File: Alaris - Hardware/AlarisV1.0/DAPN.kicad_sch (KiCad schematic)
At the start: 35 parts, among them J1 MSD-1-A, J4 Header 4x2, J5 MSD-1-A, SW3 SW_MEC_5G, SW4 SW_MEC_5G, U13 STM32H723VGTx, Y6 32k768, Y7 25MHz

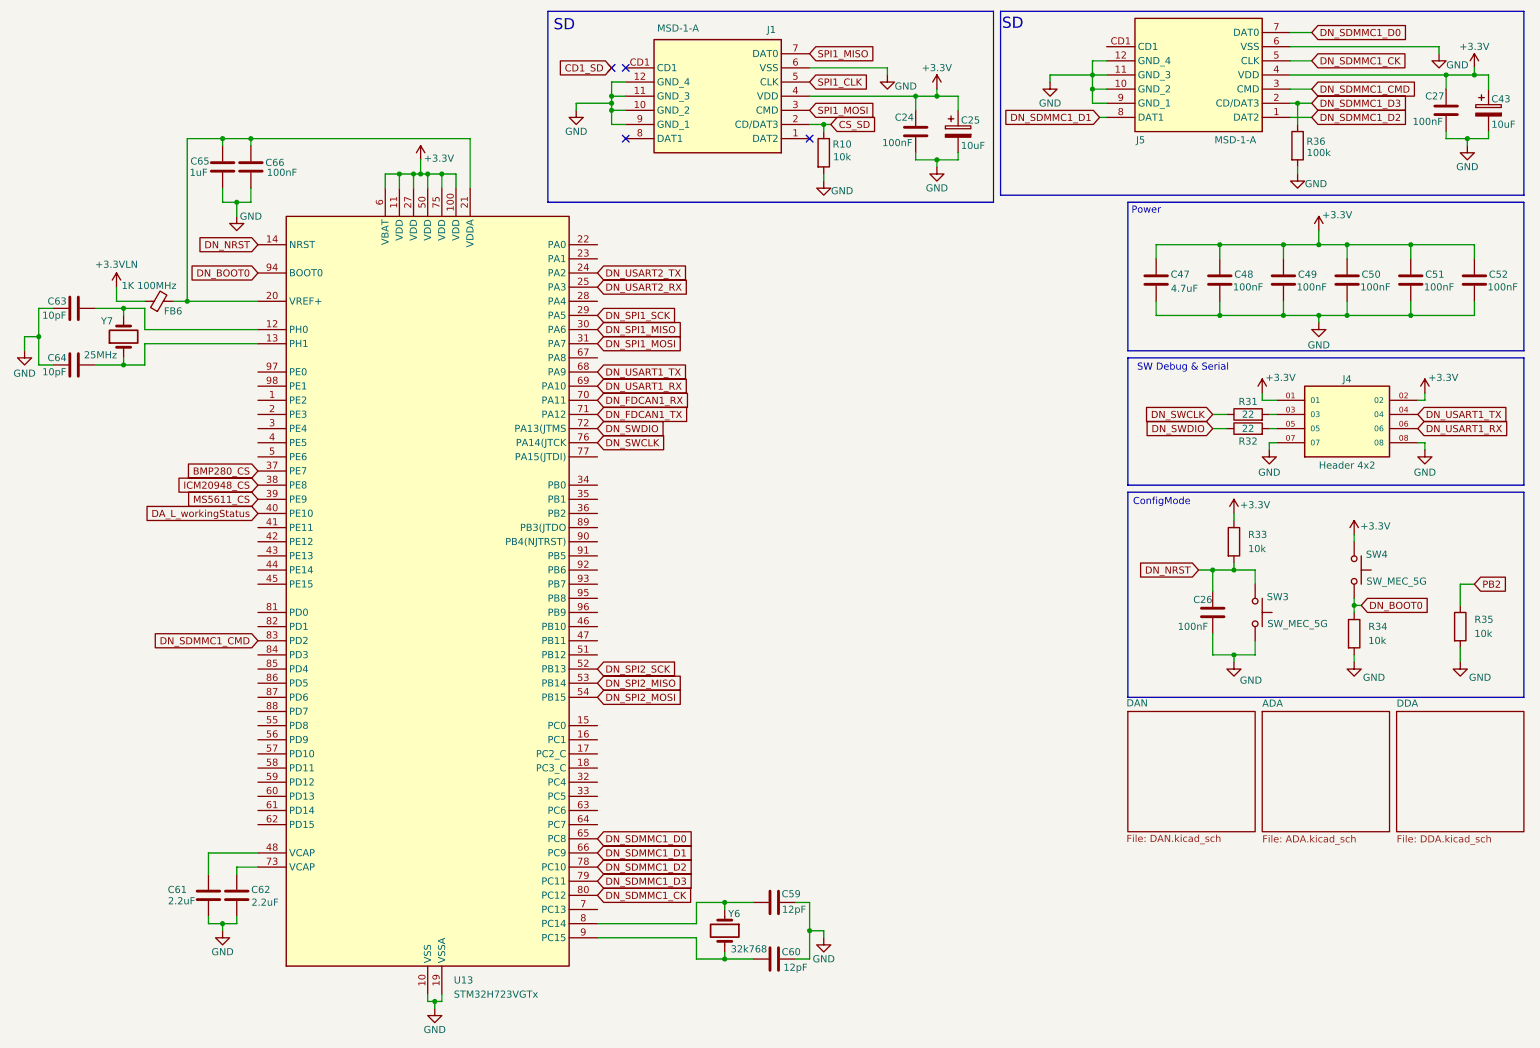
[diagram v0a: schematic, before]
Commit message: Desenvolvimento da PCB
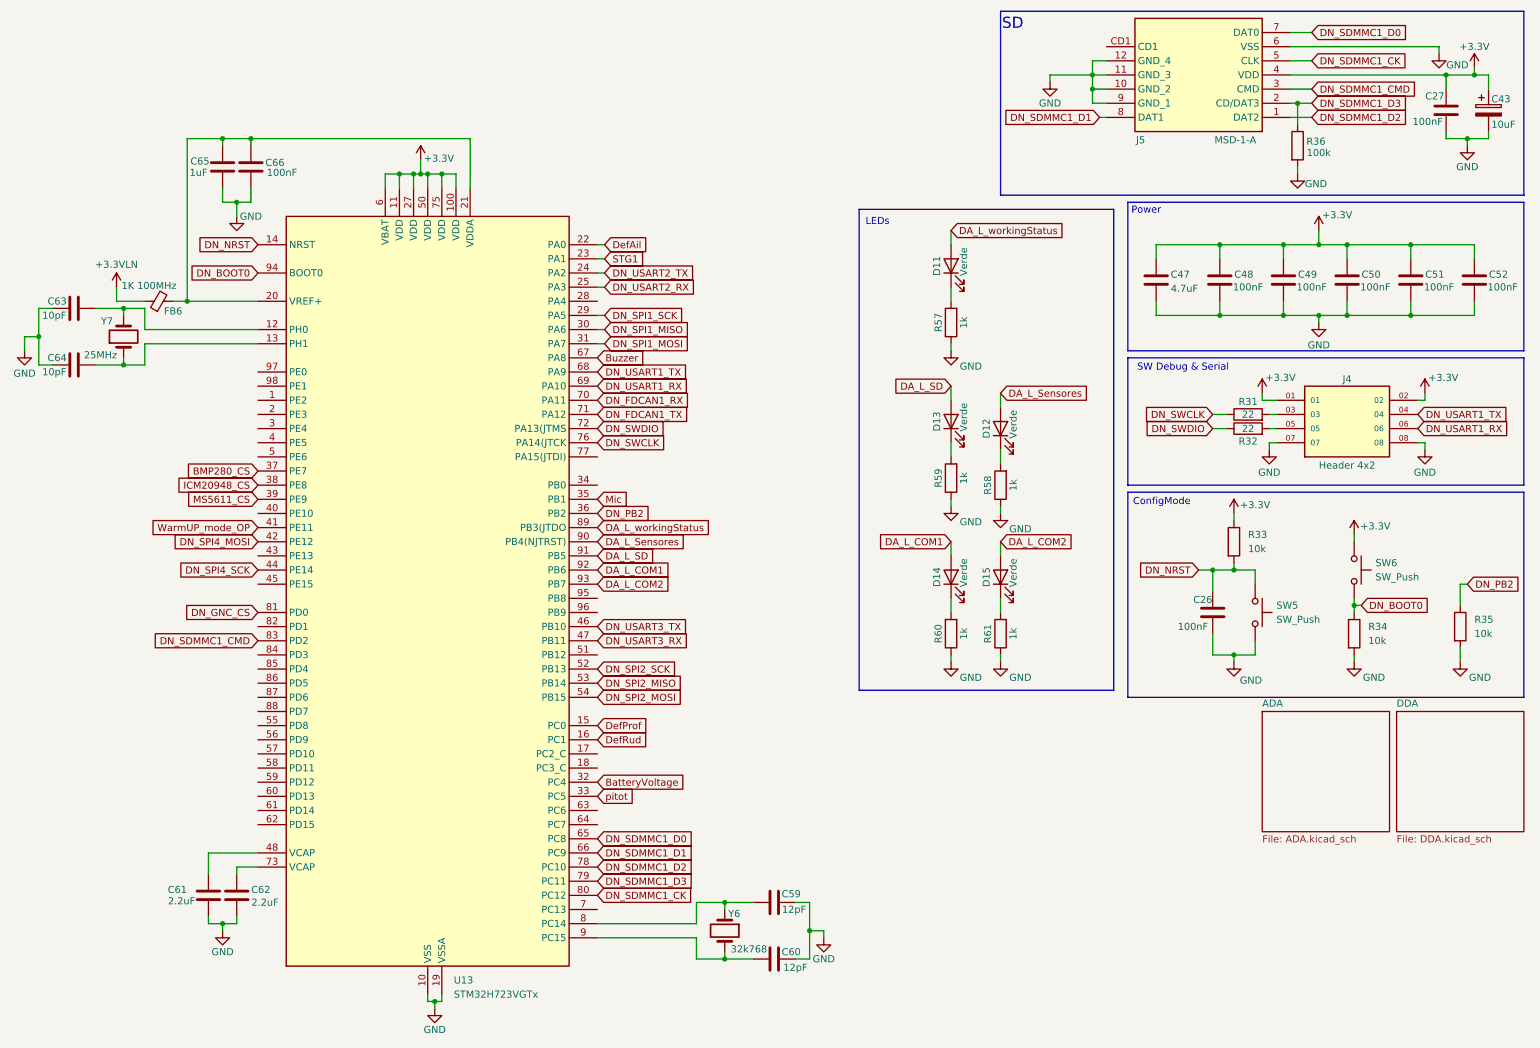
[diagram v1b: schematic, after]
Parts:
- removed C24: 100nF, Capacitor_SMD:C_0603_1608Metric_Pad1.08x0.95mm_HandSolder, symbol Device:C
- removed C25: 10uF, symbol Device:C_Polarized
- removed J1: MSD-1-A, Footprint:MSD1A, symbol MSD-1-A:MSD-1-A
- removed R10: 10k, Resistor_SMD:R_0603_1608Metric_Pad0.98x0.95mm_HandSolder, symbol Device:R
- removed SW3, SW4: SW_MEC_5G, symbol Switch:SW_MEC_5G
- added D11, D12, D13, D14, D15: Verde, LED_SMD:LED_0603_1608Metric_Pad1.05x0.95mm_HandSolder, symbol Device:LED
- added R57, R58, R59, R60, R61: 1k, Resistor_SMD:R_0603_1608Metric_Pad0.98x0.95mm_HandSolder, symbol Device:R
- added SW5, SW6: SW_Push, Footprint:SKRK, symbol Cleber:SW_Push
- C43: footprint (none) -> Capacitor_Tantalum_SMD:CP_EIA-3216-18_Kemet-A_Pad1.58x1.35mm_HandSolder
- FB6: footprint (none) -> Capacitor_SMD:C_0603_1608Metric_Pad1.08x0.95mm_HandSolder
- R31, R32: footprint (none) -> Resistor_SMD:R_0603_1608Metric_Pad0.98x0.95mm_HandSolder
- Y6: footprint Crystal:Crystal_SMD_0603-4Pin_6.0x3.5mm_HandSoldering -> Crystal:Crystal_SMD_3215-2Pin_3.2x1.5mm
- Y7: footprint Crystal:Crystal_SMD_0603-4Pin_6.0x3.5mm_HandSoldering -> Crystal:Crystal_SMD_3225-4Pin_3.2x2.5mm
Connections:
- net PB2 is gone; now on net DN_PB2: R35.1
- net +3.3V: now also SW6.1
- net DA_L_workingStatus: now also U13.89 (PB3(JTDO), D11.2 (A); no longer U13.40 (PE10)
- net DN_BOOT0: now also SW6.2
- net DN_NRST: now also SW5.1
- net GND: now also R57.1, R58.1, R59.1, R60.1, R61.1, SW5.2
- net DefProf: now reaches U13.15 (PC0)
- net DefRud: now reaches U13.16 (PC1)
- net DefAil: now reaches U13.22 (PA0)
- net STG1: now reaches U13.23 (PA1)
- net BatteryVoltage: now reaches U13.32 (PC4)
- net pitot: now reaches U13.33 (PC5)
- net Mic: now reaches U13.35 (PB1)
- net DN_PB2: now reaches U13.36 (PB2)
- net WarmUP_mode_OP: now reaches U13.41 (PE11)
- net DN_SPI4_MOSI: now reaches U13.42 (PE12)
- net DN_SPI4_SCK: now reaches U13.44 (PE14)
- net DN_USART3_TX: now reaches U13.46 (PB10)
- net DN_USART3_RX: now reaches U13.47 (PB11)
- net Buzzer: now reaches U13.67 (PA8)
- net DN_GNC_CS: now reaches U13.81 (PD0)
- net DA_L_Sensores: now reaches U13.90 (PB4(NJTRST))
- net DA_L_Sensores: now also D12.2 (A)
- net DA_L_SD: now reaches U13.91 (PB5)
- net DA_L_SD: now also D13.2 (A)
- net DA_L_COM1: now reaches U13.92 (PB6)
- net DA_L_COM1: now also D14.2 (A)
- net DA_L_COM2: now reaches U13.93 (PB7)
- net DA_L_COM2: now also D15.2 (A)
- new net: D14.1 (K), R60.2
- new net: D11.1 (K), R57.2
- new net: D12.1 (K), R58.2
- new net: D15.1 (K), R61.2
- new net: D13.1 (K), R59.2
- no-connect marks 4 -> 0
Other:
- removed sheet DAN
- note added: "LEDs"
